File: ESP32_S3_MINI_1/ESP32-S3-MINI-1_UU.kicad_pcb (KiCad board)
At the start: 2 copper layers, 20.3 x 45.7 mm, 54 parts, among them IC1 TPS6282533DMQR, IC2 BQ25185DLHR, J1 JST_2mm_LiPo, J2 USB4120-03-C, J3 Qwiic_Vertical, J4 Castellated_1x01, J7 Castellated_1x01, J8 Castellated_1x16, J9 Castellated_1x18, U1 LM66100DCK, U2 ESP32-S3-MINI-1, U3 MAX17048, U4 TMP102, U5 LM66100DCK

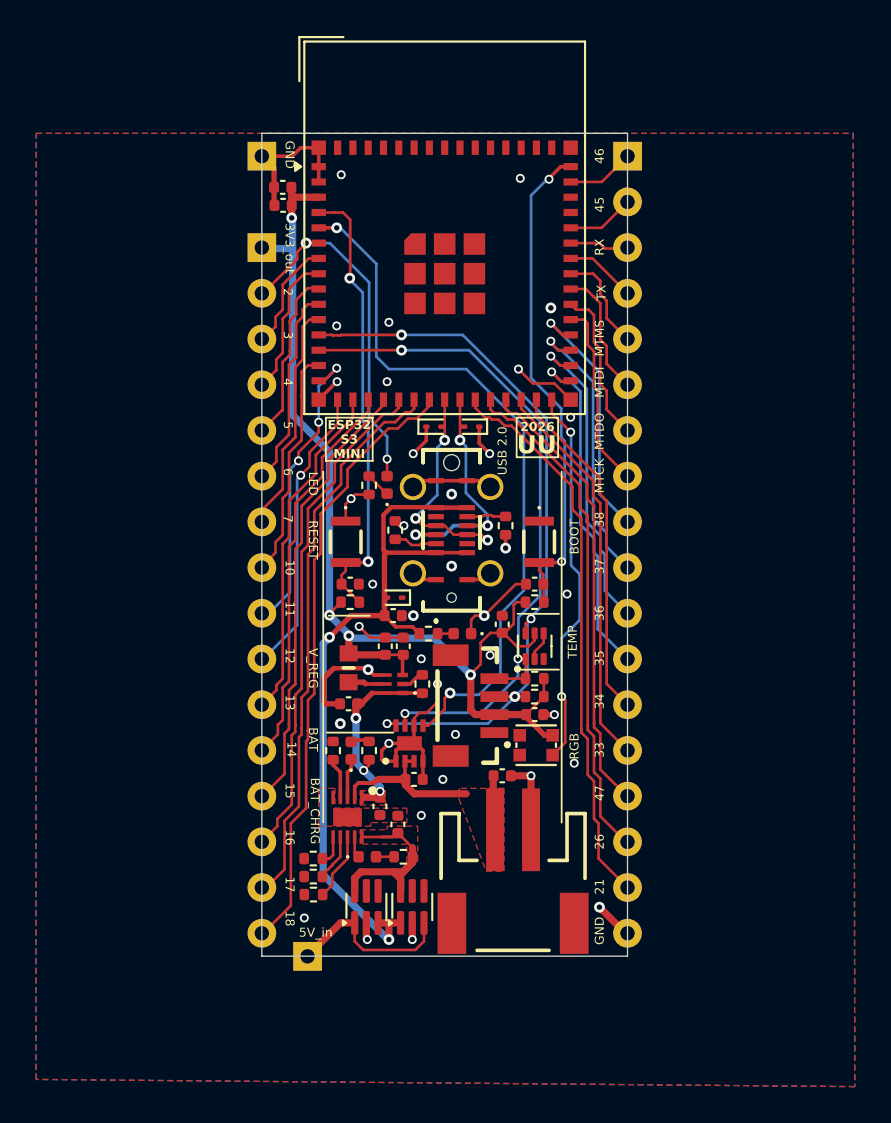
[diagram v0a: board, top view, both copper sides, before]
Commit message: Trace cleanup
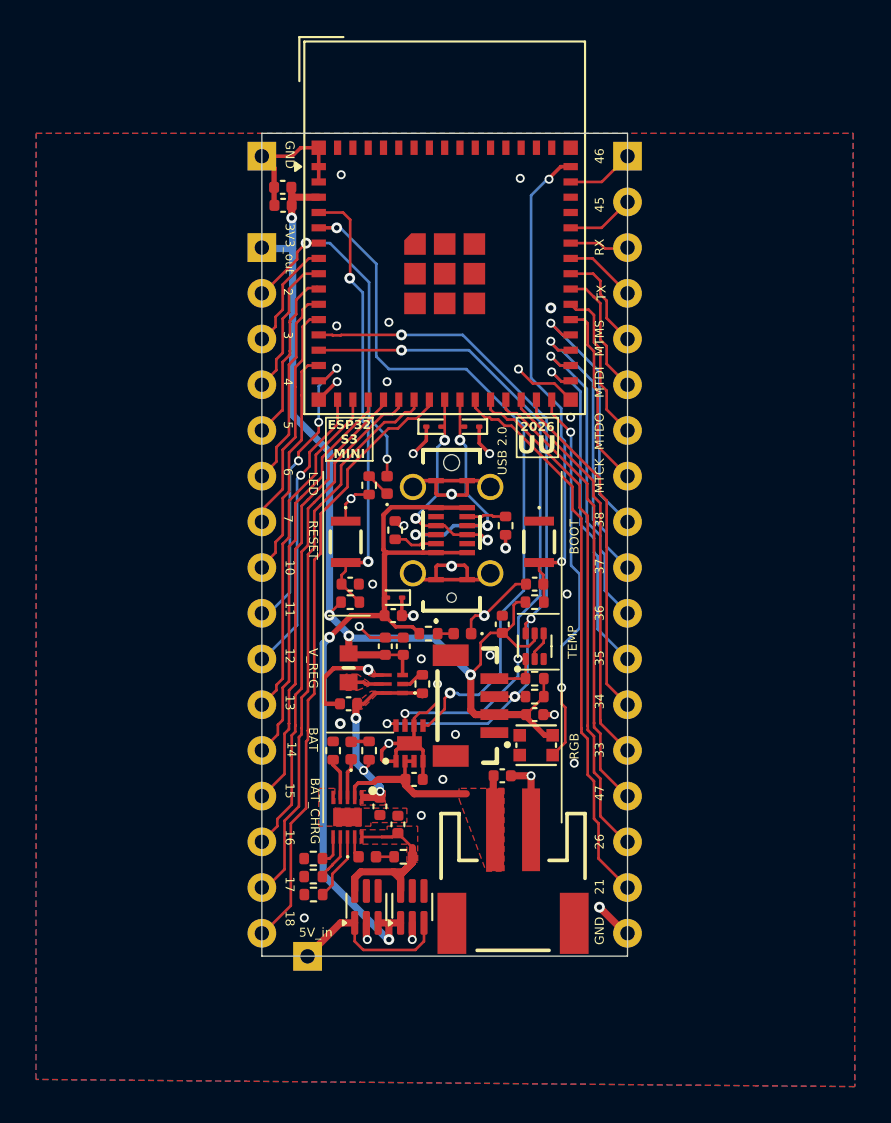
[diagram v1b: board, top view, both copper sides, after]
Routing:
- net GND: track 63.1 -> 72.7 mm
- added copper zone on F.Cu, net Net-(IC1-SW)
